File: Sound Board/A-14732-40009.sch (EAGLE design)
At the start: 234 parts, among them P2 AUX IN, P3 AUX OUT, P4 ORKIN R/W, P5 VOLUME, Q1 MPS3646, U1 OKI6295, U10 26LS32A, U11 26LS31, U12 27C040-150, U13 27C040-150, U14 YAMAHA 2151, U15 TIL7524, U16 74LS374, U17 74LS174, U18 16L8, U19 74LS11, U2 2064, U20 74LS139, U21 74LS14, U22 74LS74, U23 74LS74, U24 26LS31, U25 26LS32A, U26 74LS04, U28 YAMAHA 3012, U29 LM324D, U3 27C040, U30 MC3340, U31 HA3116, U32 TL084D, U33 TL084D, U4 6809E, U5 74LS374DW, U6 26LS32A, U7 26LS31, U8 74LS138, U9 74LS74, Y1 3.5749MHz, Y2 8MHz

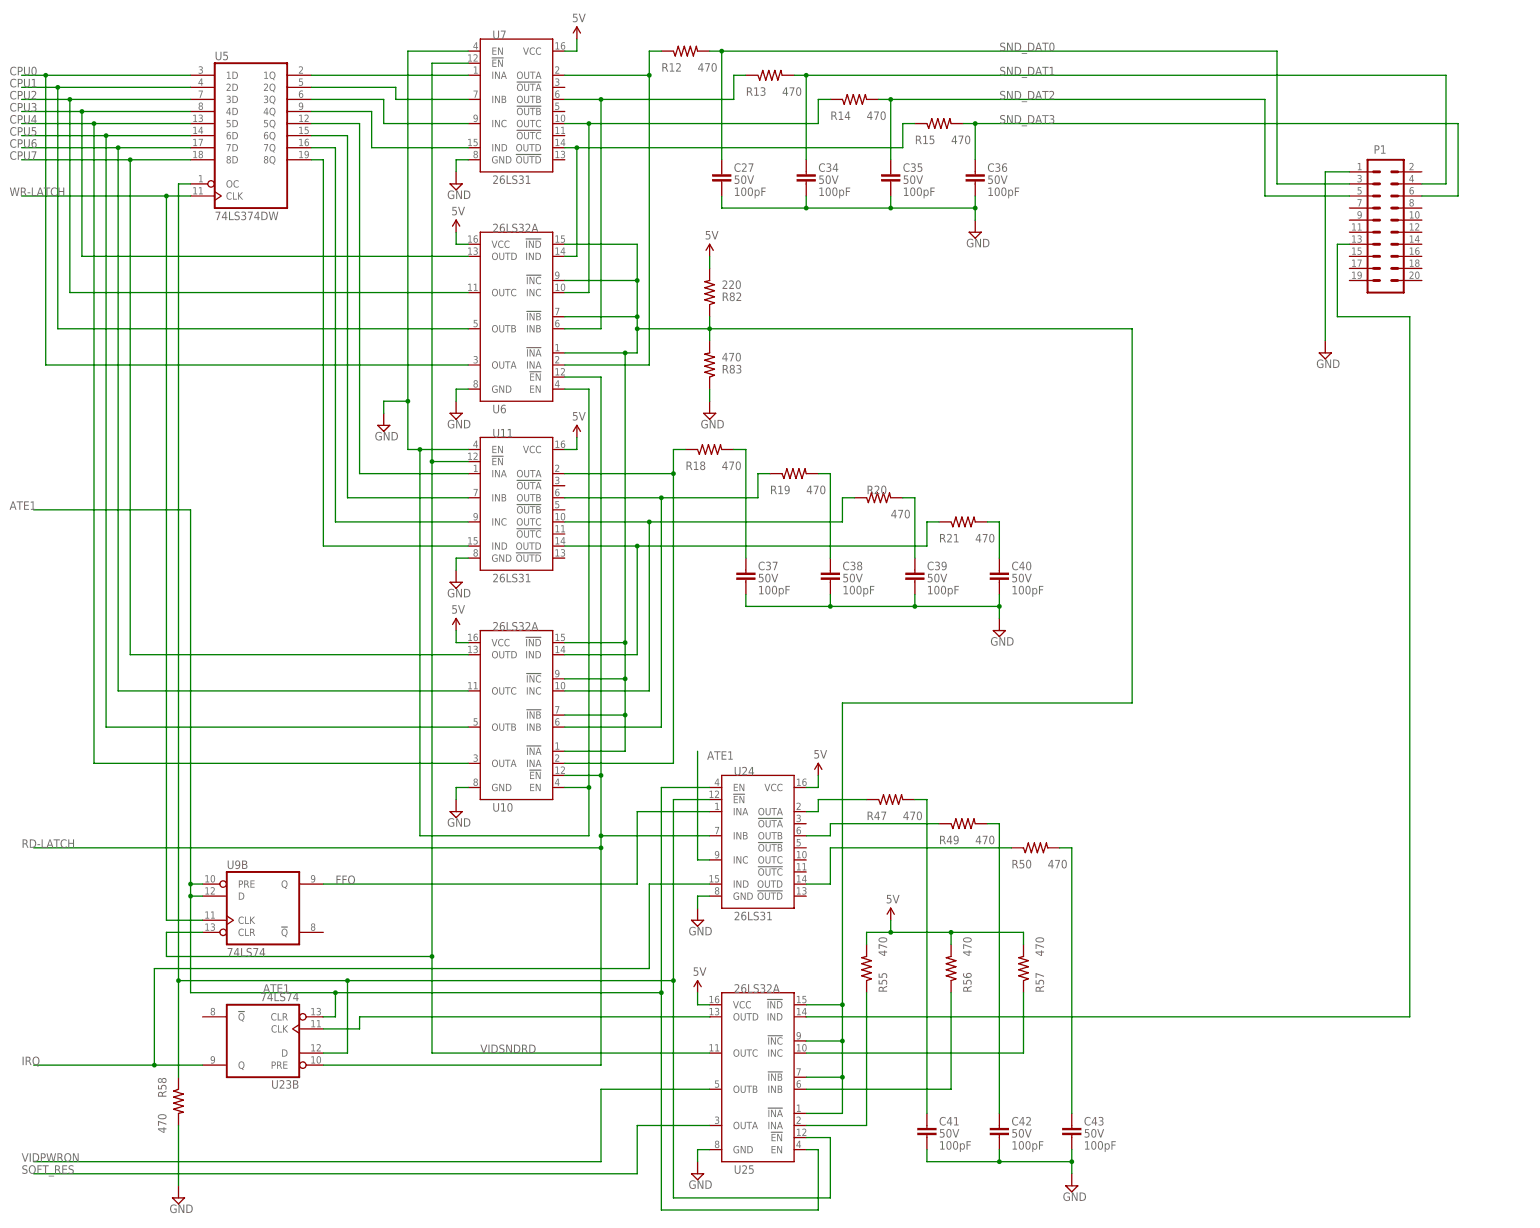
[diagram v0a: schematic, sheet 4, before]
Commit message: P1 connected mostly wired up
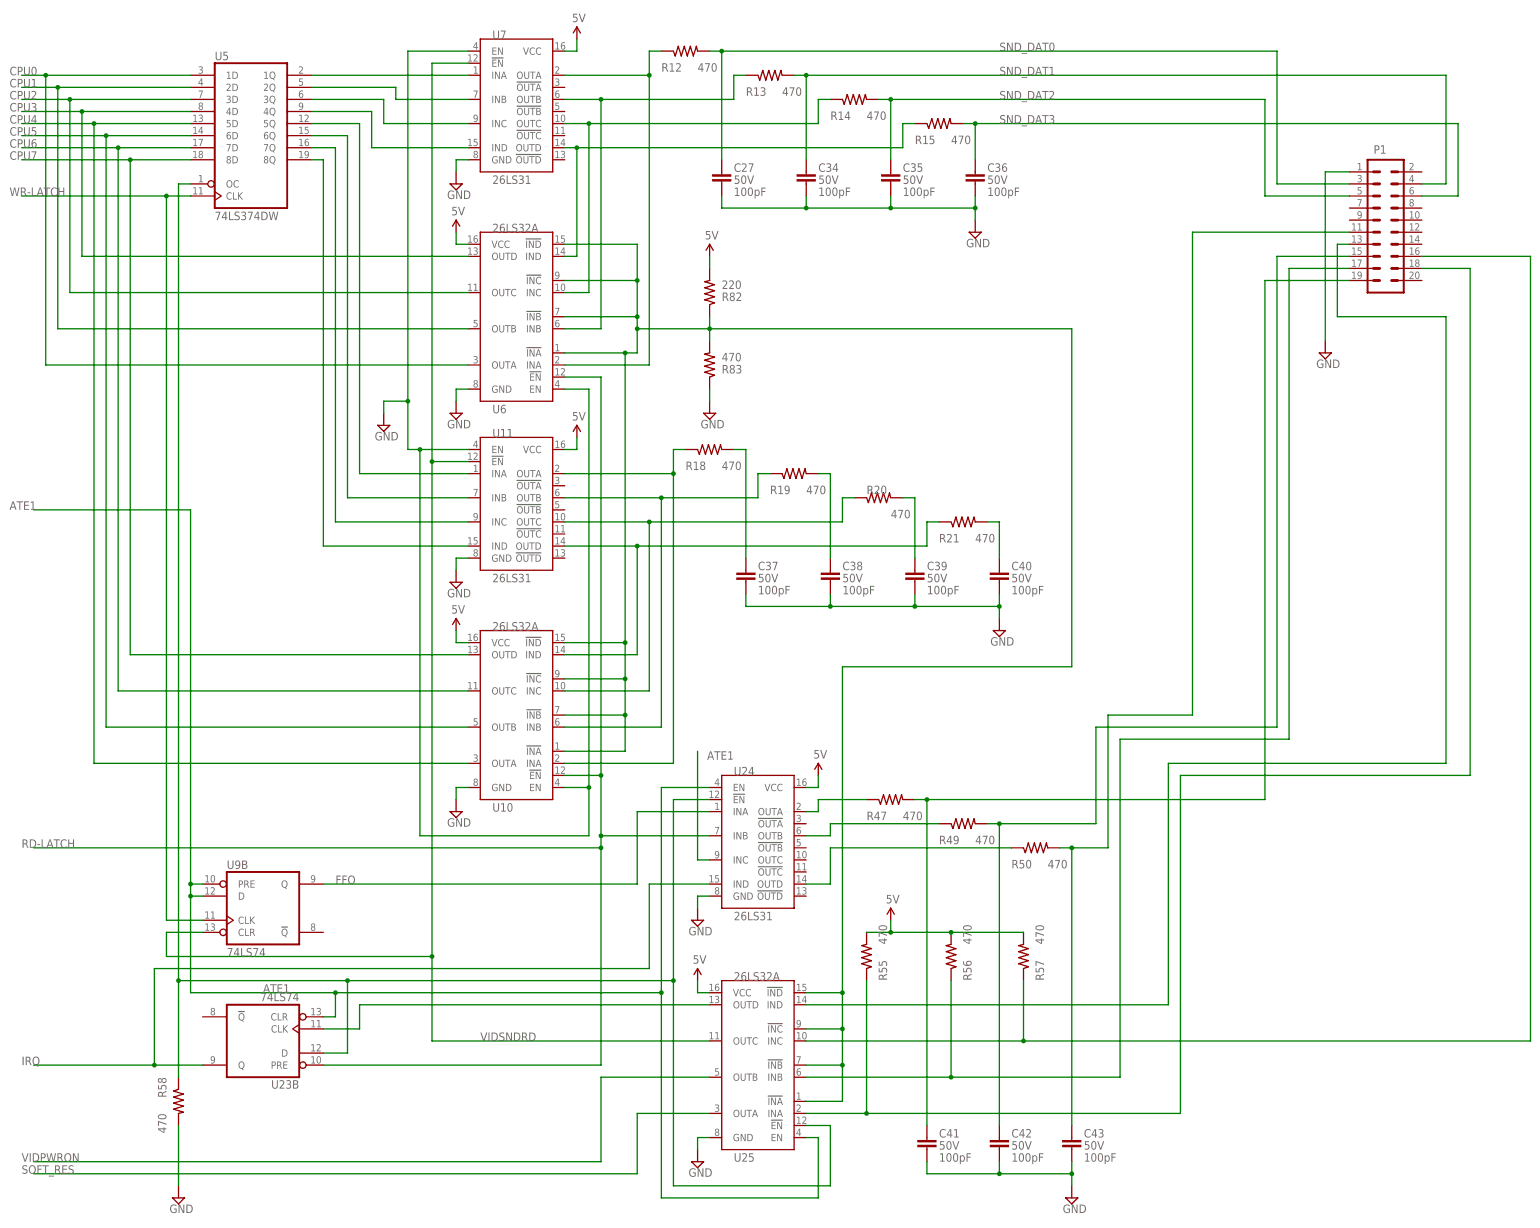
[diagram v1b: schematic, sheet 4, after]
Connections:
- net N$129: now also P1.19
- net N$130: now also P1.15
- net N$131: now also P1.11
- net N$132: now also P1.18
- net N$133: now also P1.17
- net N$134: now also P1.16
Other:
- moved on the sheet: C41, C42, C43, R55, R56, R57, U25
